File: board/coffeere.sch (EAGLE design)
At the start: 14 parts

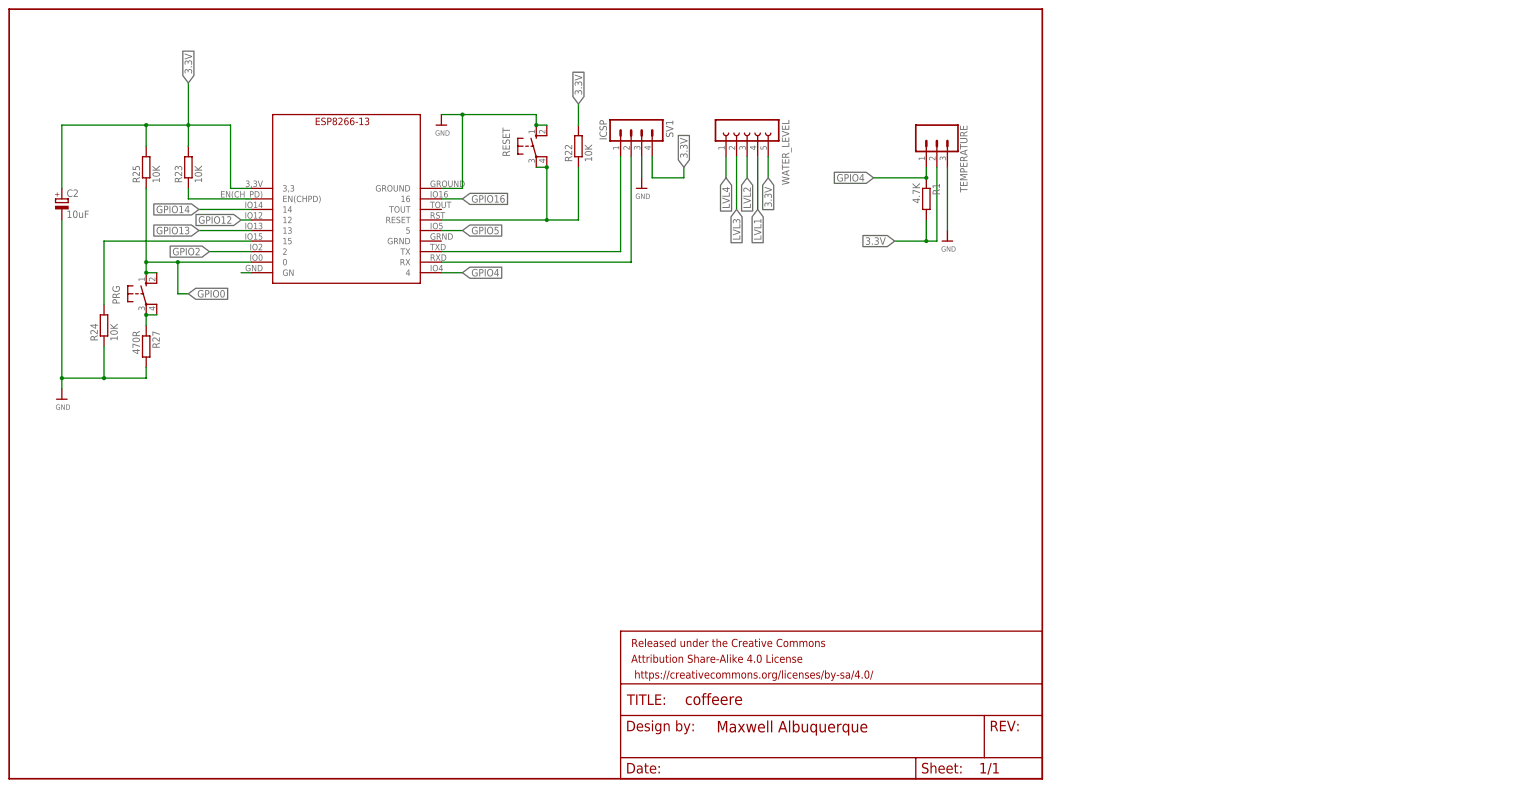
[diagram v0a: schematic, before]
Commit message: Creating schemetic and board designs.
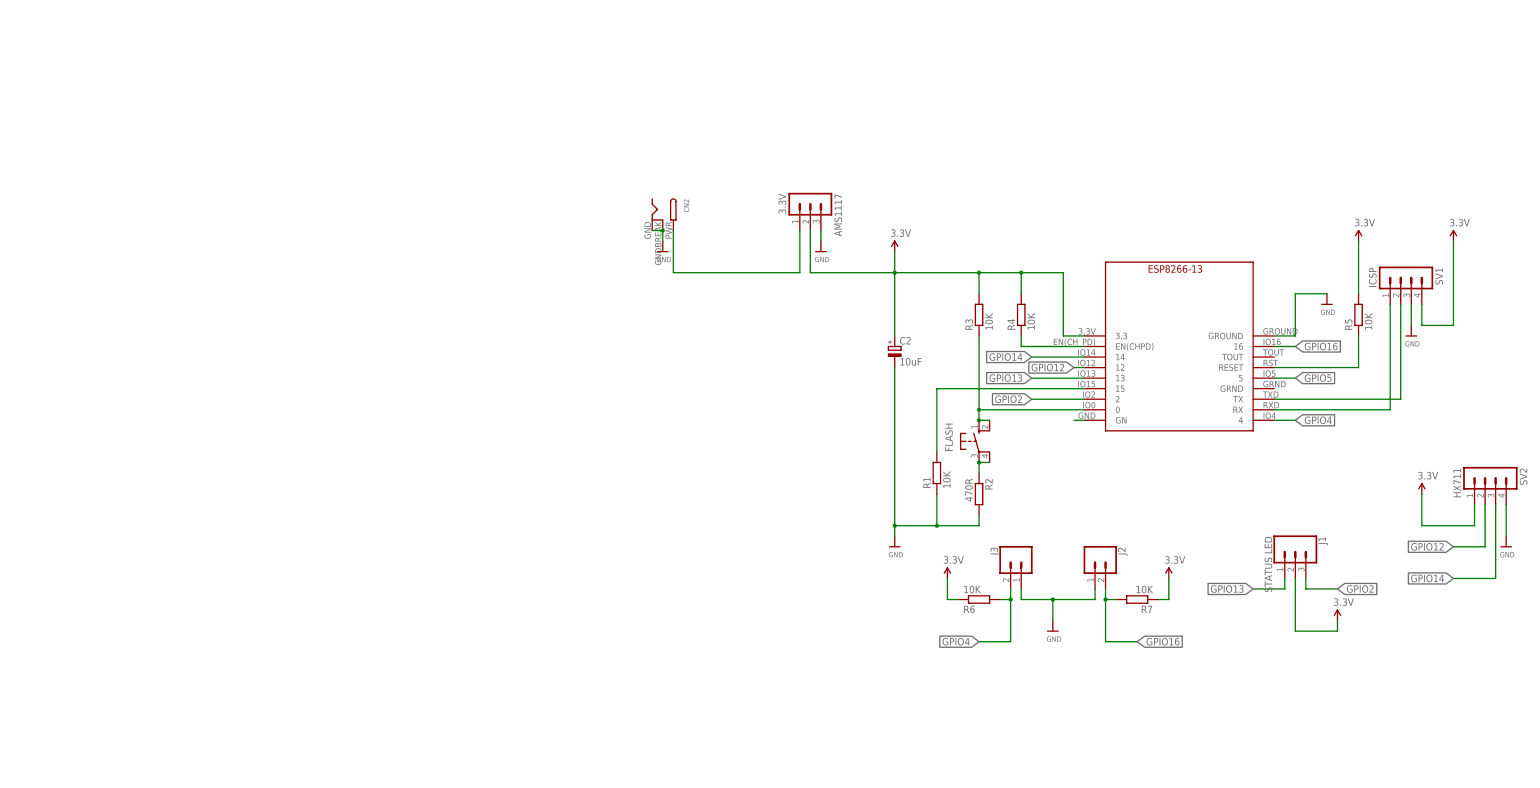
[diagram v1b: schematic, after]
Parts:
- removed FRAME2: FRAME-LETTER, SparkFun-Aesthetics:FRAME-LETTER
- removed PRG, RESET: (no value), switch-omron:10-XX
- removed R22, R23, R24, R25: 10K, rcl:R-EU_0207/10
- removed R27: 470R, rcl:R-EU_0207/10
- removed TEMPERATURE: (no value), SparkFun-Connectors:CONN_03
- removed WATER_LEVEL: (no value), con-lsta:FE05-1
- added AMS1117: 3.3V, con-lstb:MA03-1
- added CN2: (no value), adafruit:DCBARRELPTH
- added FLASH: (no value), switch-omron:10-XX
- added J1: STATUS LED, SparkFun-Connectors:CONN_03
- added J2, J3: (no value), SparkFun-Connectors:CONN_02
- added R2: 470R, rcl:R-EU_0207/10
- added R3, R4, R5, R6, R7: 10K, rcl:R-EU_0207/10
- added SV2: HX711, con-lstb:MA04-1
- R1: value 4.7K -> 10K
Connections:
- removed net LVL1: WATER_LEVEL.4
- removed net LVL2: WATER_LEVEL.3
- removed net LVL3: WATER_LEVEL.2
- removed net LVL4: WATER_LEVEL.1
- new net N$2: AMS1117.1, CN2.PWR
- net 3.3V: now also AMS1117.2, J1.2, R3.2, R4.2, R5.2, R6.1, R7.1, SV2.1; no longer R1.2, R22.2, R23.2, R25.2, TEMPERATURE.2, WATER_LEVEL.5
- net GND: now also AMS1117.3, CN2.GND, CN2.GNDBREAK, J2.1, J3.1, R1.1, R2.2, SV2.4; no longer R24.1, R27.2, RESET.S, RESET.S1, TEMPERATURE.3
- net GPIO0: now also FLASH.S, FLASH.S1, R3.1; no longer PRG.S, PRG.S1, R25.1
- net GPIO12: now also SV2.2
- net GPIO13: now also J1.1
- net GPIO14: now also SV2.3
- net GPIO15: now also R1.2; no longer R24.2
- net GPIO16: now also J2.2, R7.2
- net GPIO2: now also J1.3
- net GPIO4: now also J3.2, R6.2; no longer R1.1, TEMPERATURE.1
- net N$12: now also SV1.2; no longer SV1.1
- net N$13: now also SV1.1; no longer SV1.2
- net N$15: now also FLASH.P, FLASH.P1, R2.1; no longer PRG.P, PRG.P1, R27.1
- net N$16: now also R5.1; no longer R22.1, RESET.P, RESET.P1
- net N$17: now also R4.1; no longer R23.1
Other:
- moved on the sheet: C2, R1, SV1
